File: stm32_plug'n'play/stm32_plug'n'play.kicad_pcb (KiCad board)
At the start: 4 copper layers, 60.2 x 38.4 mm, 48 parts, among them J1 Screw_Terminal_01x02, J2 USB_B_Micro, SW1 SW_SPDT, U1 STM32F302C8Tx, U2 AMS1117-3.3, U3 BMP388, U4 MPU-6050, U5 TMP112, Y1 X322516MLB4SI

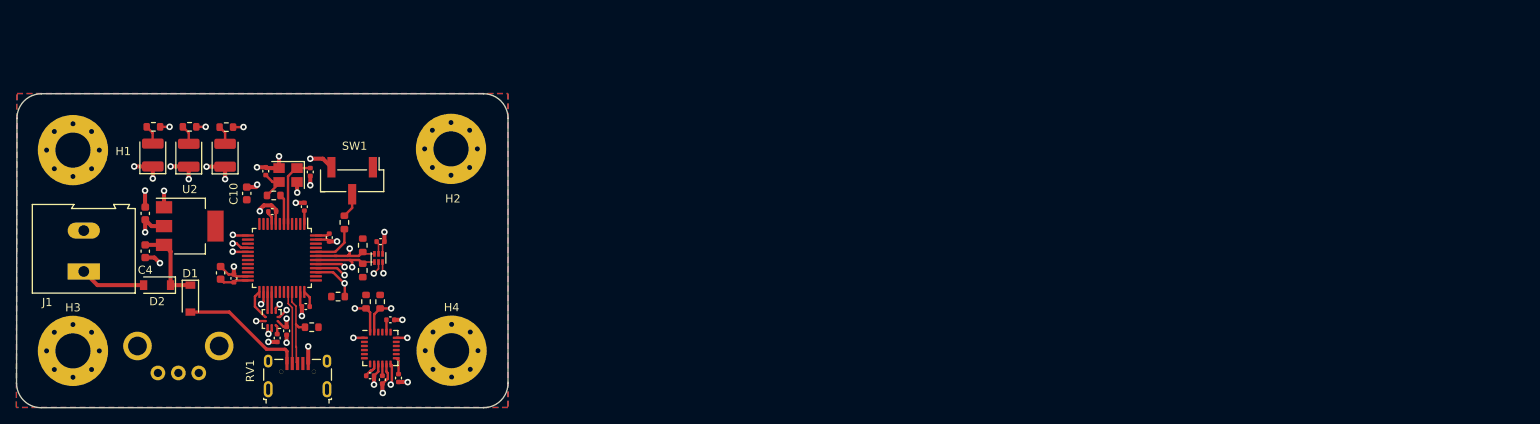
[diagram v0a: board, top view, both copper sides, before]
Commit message: Add files via upload
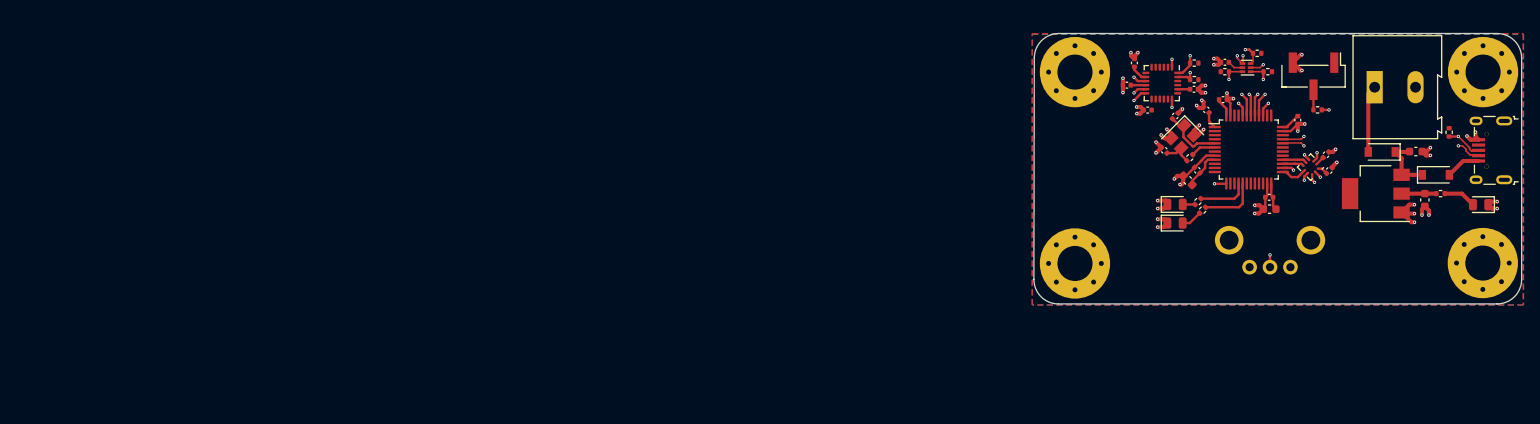
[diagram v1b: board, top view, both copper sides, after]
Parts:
- D3, D4, D5: footprint LED_SMD:LED_1210_3225Metric -> LED_SMD:LED_0805_2012Metric
- R1, R10, R11, R2, R3, R4, R5, R6, R7, R8, R9: footprint Resistor_SMD:R_0603_1608Metric -> Resistor_SMD:R_0402_1005Metric
- moved H3 172.9 mm to (199.8, 83.0)
- moved H1 172.9 mm to (199.8, 59.6)
- moved J1 159.6 mm to (186.6, 61.5), turned to 0 degrees
- moved C7 156.6 mm to (192.7, 75.3), turned to 90 degrees
- moved C4 156.0 mm to (191.6, 69.4), turned to 180 degrees
- moved D3 153.8 mm to (199.5, 75.9), turned to 180 degrees
- moved D1 153.2 mm to (194.1, 72.2), turned to 0 degrees
- moved D2 150.8 mm to (187.4, 69.4)
- moved R1 148.8 mm to (194.6, 74.5), turned to 180 degrees
- moved J2 148.3 mm to (200.7, 69.0), turned to 90 degrees
- moved U2 145.2 mm to (186.7, 74.5), turned to 180 degrees
- moved R2 141.3 mm to (195.7, 67.0), turned to 90 degrees
- moved RV1 134.3 mm to (171.5, 83.3)
- moved C3 131.7 mm to (177.2, 65.5), turned to -90 degrees
- moved C13 130.4 mm to (181.0, 71.7), turned to -135 degrees
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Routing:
- net +3V3: track 85.7 -> 25.7 mm, vias 3 -> 0
- net /Alert_Notif: track 26.7 -> 7.18 mm, vias 2 -> 0
- net /RV_In: track 21.5 -> 2.97 mm, vias 1 -> 2
- net /USB_D+: track 10.3 -> 26.4 mm, vias 0 -> 2
- net /USB_D-: track 8.98 -> 25.0 mm, vias 0 -> 2
- net /PWM_Out: track 19.8 -> 6.16 mm, vias 2 -> 0
- net /SDA0: track 30.7 -> 19.0 mm, vias 2 -> 3
- net GND: track 68.5 -> 79.8 mm, vias 33 -> 56
- net VBUS: track 15.3 -> 4.27 mm
- net /MPU_INT: track 25.1 -> 21.0 mm
- net /Boot_Mode: track 5.61 -> 2.61 mm, vias 0 -> 2
- net /SCL0: track 22.5 -> 19.6 mm, vias 2 -> 3
- net Net-(C4-Pad2): track 9.98 -> 7.79 mm
- net Net-(D3-Pad2): track 2.32 -> 4.06 mm
- net /Crystal_In: track 8.98 -> 7.65 mm
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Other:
- board size 60.2 x 38.4 mm -> 59.7 x 33.1 mm
- board text added: "JLCJLCJLCJLC"

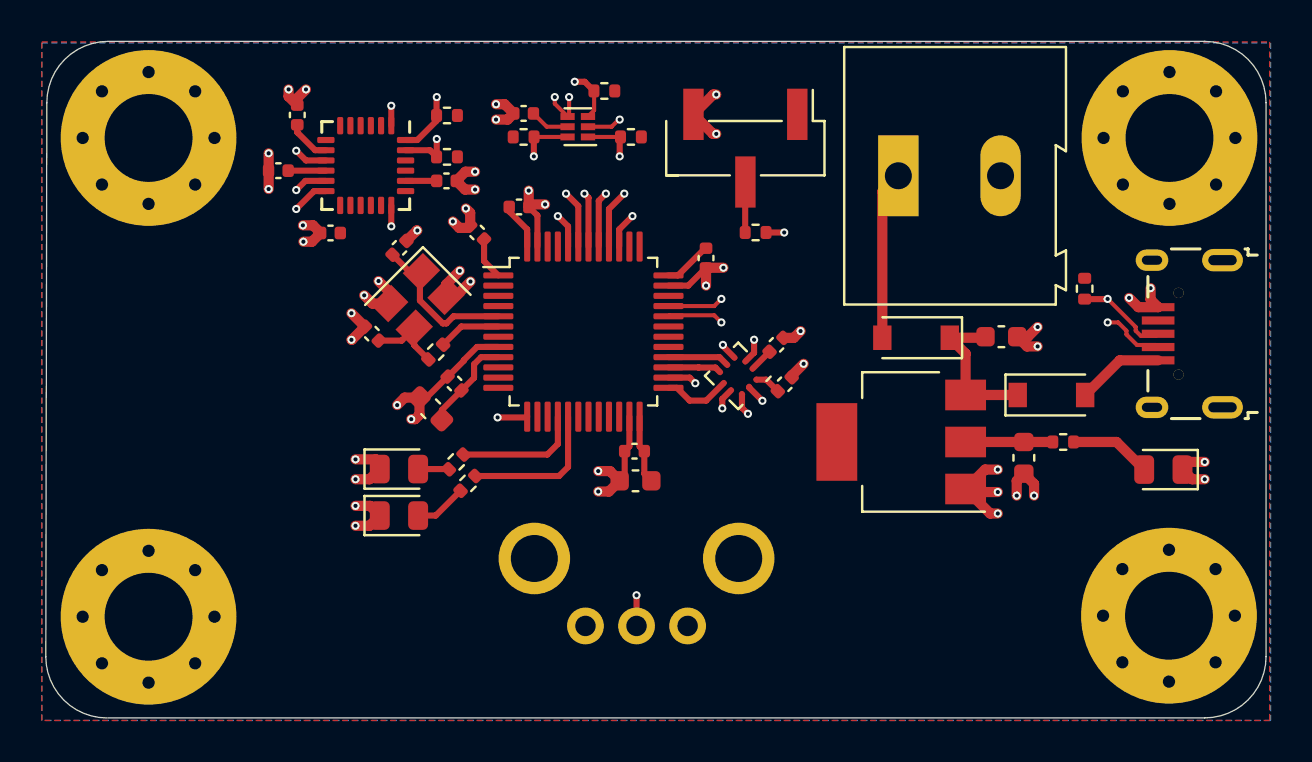
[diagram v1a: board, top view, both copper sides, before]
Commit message: Add files via upload
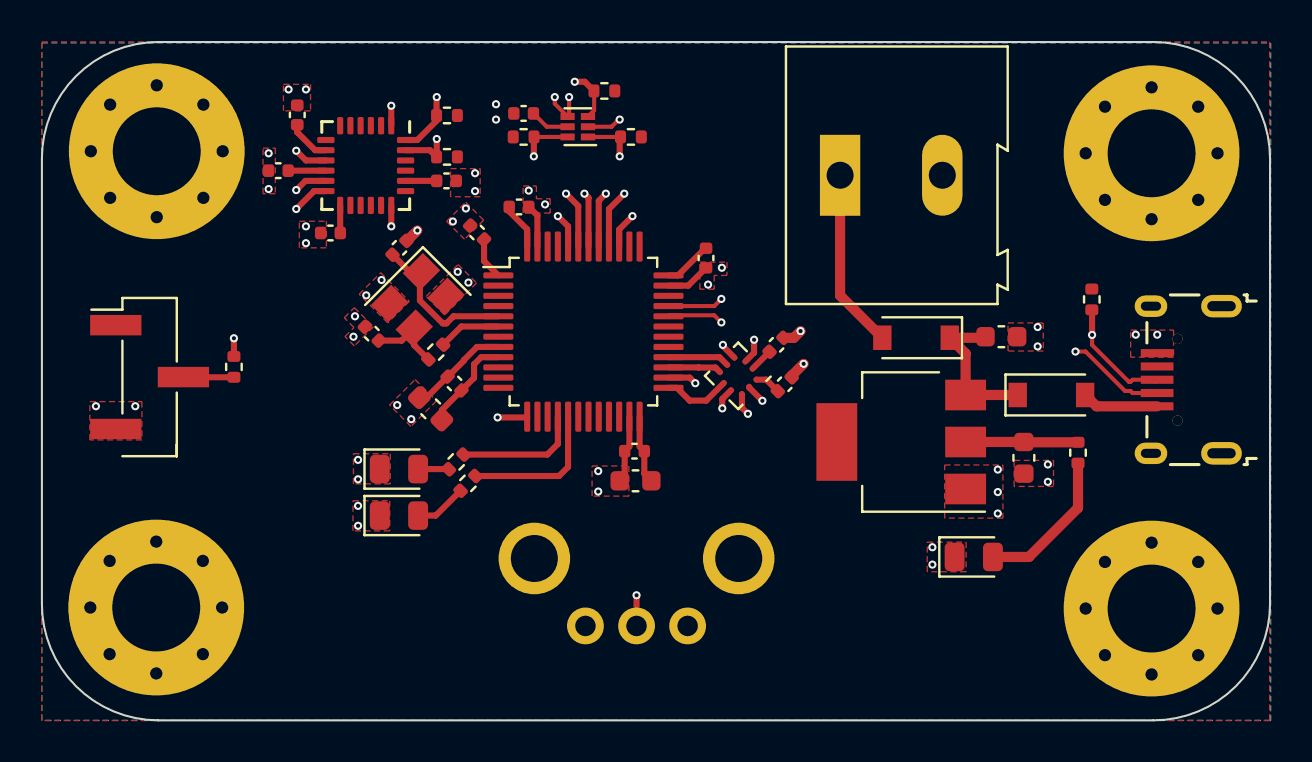
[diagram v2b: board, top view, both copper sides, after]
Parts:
- moved SW1 31.2 mm to (149.9, 71.3), turned to 0 degrees
- moved R11 26.4 mm to (154.1, 70.8), turned to -90 degrees
- moved D3 10.2 mm to (190.2, 80.2), turned to 0 degrees
- moved J1 2.85 mm to (183.7, 61.5)
- moved J2 2.25 mm to (200.6, 71.2)
- moved H1 1.15 mm to (198.9, 60.4)
- moved H3 0.92 mm to (198.9, 82.7)
- moved R1 0.90 mm to (195.3, 75.0), turned to 90 degrees
- moved H2 0.76 mm to (150.3, 60.3)
- moved R2 0.63 mm to (196.0, 67.5)
- moved H4 0.59 mm to (150.2, 82.6)
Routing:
- net GND: track 79.8 -> 27.8 mm
- net /Boot_Mode: track 2.61 -> 21.3 mm
- net /RV_In: track 2.97 -> 14.5 mm
- net Net-(D3-Pad2): track 4.06 -> 7.40 mm
- net +3V3: track 25.7 -> 28.2 mm
- net /USB_D-: track 25.0 -> 26.2 mm
- net /USB_D+: track 26.4 -> 27.5 mm
- net +BATT: track 8.25 -> 8.81 mm
- net VBUS: track 4.27 -> 3.75 mm
- added copper zone on F.Cu, net GND
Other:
- board size 59.7 x 33.1 mm -> 60.1 x 33.2 mm

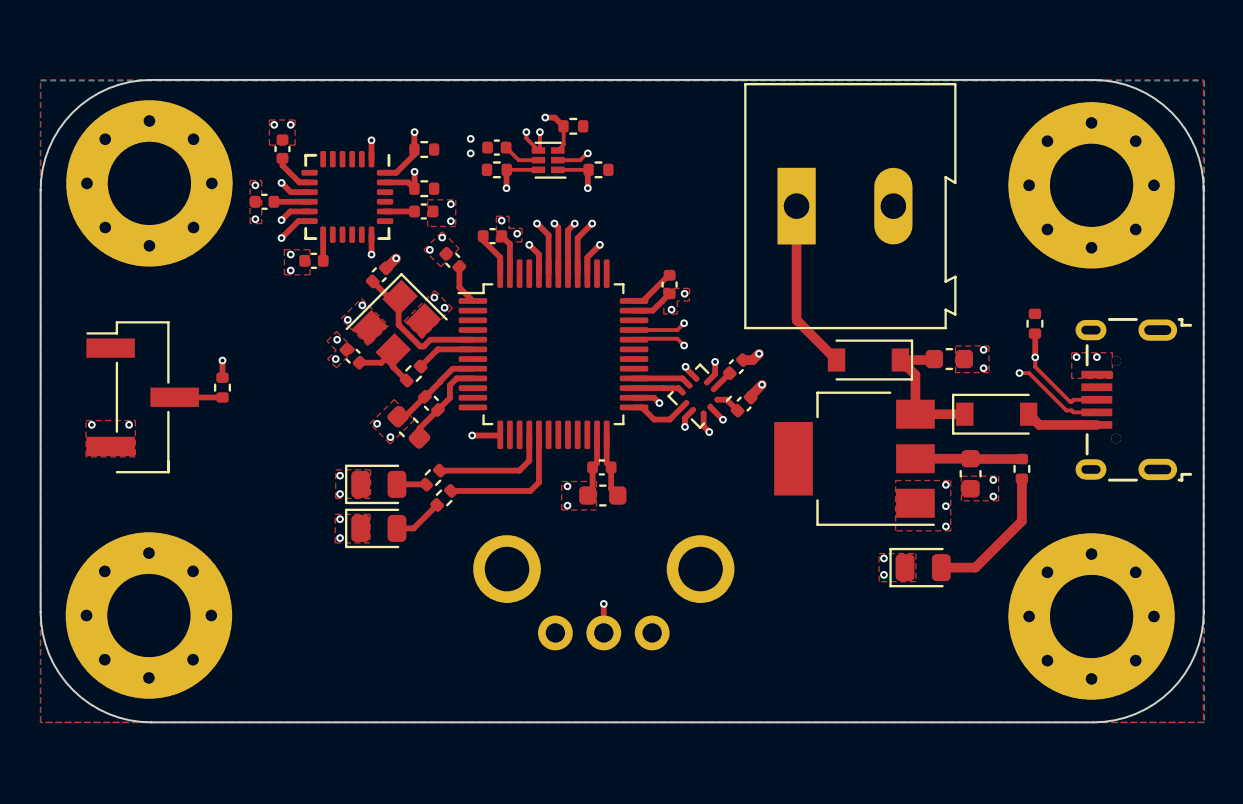
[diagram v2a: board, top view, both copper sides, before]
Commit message: Add files via upload
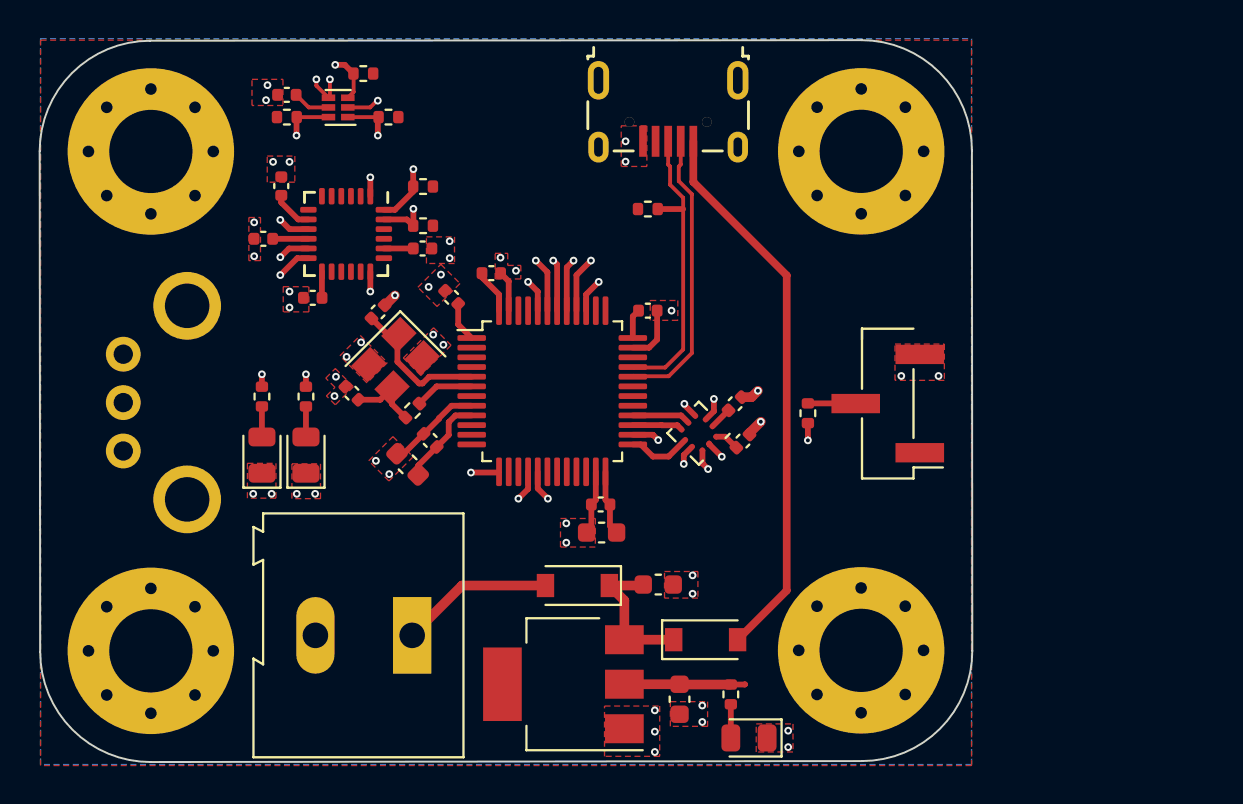
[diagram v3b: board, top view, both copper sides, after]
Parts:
- removed H1, H2, H3: MountingHole_Pad, MountingHole:MountingHole_4.3mm_M4_Pad_Via
- added H4: MountingHole_Pad, MountingHole:MountingHole_4.3mm_M4_Pad_Via, F.Cu at (187.1, 58.6)
- added H4: MountingHole_Pad, MountingHole:MountingHole_4.3mm_M4_Pad_Via, F.Cu at (187.0, 84.4)
- added H4: MountingHole_Pad, MountingHole:MountingHole_4.3mm_M4_Pad_Via, F.Cu at (150.3, 58.6)
- moved SW1 38.5 mm to (188.4, 71.7), turned to 180 degrees
- moved R11 30.3 mm to (184.3, 72.2), turned to 90 degrees
- moved J1 29.8 mm to (163.8, 83.7), turned to 180 degrees
- moved J2 27.9 mm to (176.8, 56.7), turned to 180 degrees
- moved RV1 26.3 mm to (149.2, 69.4), turned to 180 degrees
- moved R2 20.9 mm to (176.0, 61.6), turned to 180 degrees
- moved D1 19.0 mm to (179.0, 83.9)
- moved D2 19.0 mm to (172.4, 81.1)
- moved C4 19.0 mm to (176.6, 81.0)
- moved C7 19.0 mm to (177.7, 87.0)
- moved R1 19.0 mm to (180.3, 86.7)
- moved U2 19.0 mm to (171.7, 86.2)
- moved D3 12.6 mm to (181.3, 89.0), turned to 180 degrees
- moved R8 11.2 mm to (161.3, 54.6)
- moved R10 11.2 mm to (157.4, 56.9)
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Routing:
- net VBUS: track 3.75 -> 28.8 mm
- net /USB_D+: track 27.5 -> 15.4 mm, vias 2 -> 0
- net /PWM_Out: track 6.16 -> 18.1 mm, vias 0 -> 2
- net /Temp_ALERT: track 12.1 -> 23.8 mm
- net /USB_D-: track 26.2 -> 14.9 mm, vias 2 -> 0
- net /Alert_Notif: track 7.18 -> 17.7 mm, vias 0 -> 2
- net /SDA0: track 19.0 -> 25.6 mm
- net /RV_In: track 14.5 -> 20.9 mm, vias 2 -> 1
- net Net-(D3-Pad2): track 7.40 -> 1.79 mm
- net Net-(D5-Pad2): track 2.58 -> 1.58 mm
- net +BATT: track 8.81 -> 7.95 mm
- net GND: track 27.8 -> 28.6 mm, vias 56 -> 55
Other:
- board size 60.1 x 33.2 mm -> 48.2 x 37.3 mm
